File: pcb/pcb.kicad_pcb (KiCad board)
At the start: 2 copper layers, 108.7 x 45.2 mm, 22 parts, among them SW1 SW_Push, U1 ATmega32U4-AU, Y1 Crystal_GND24_Small

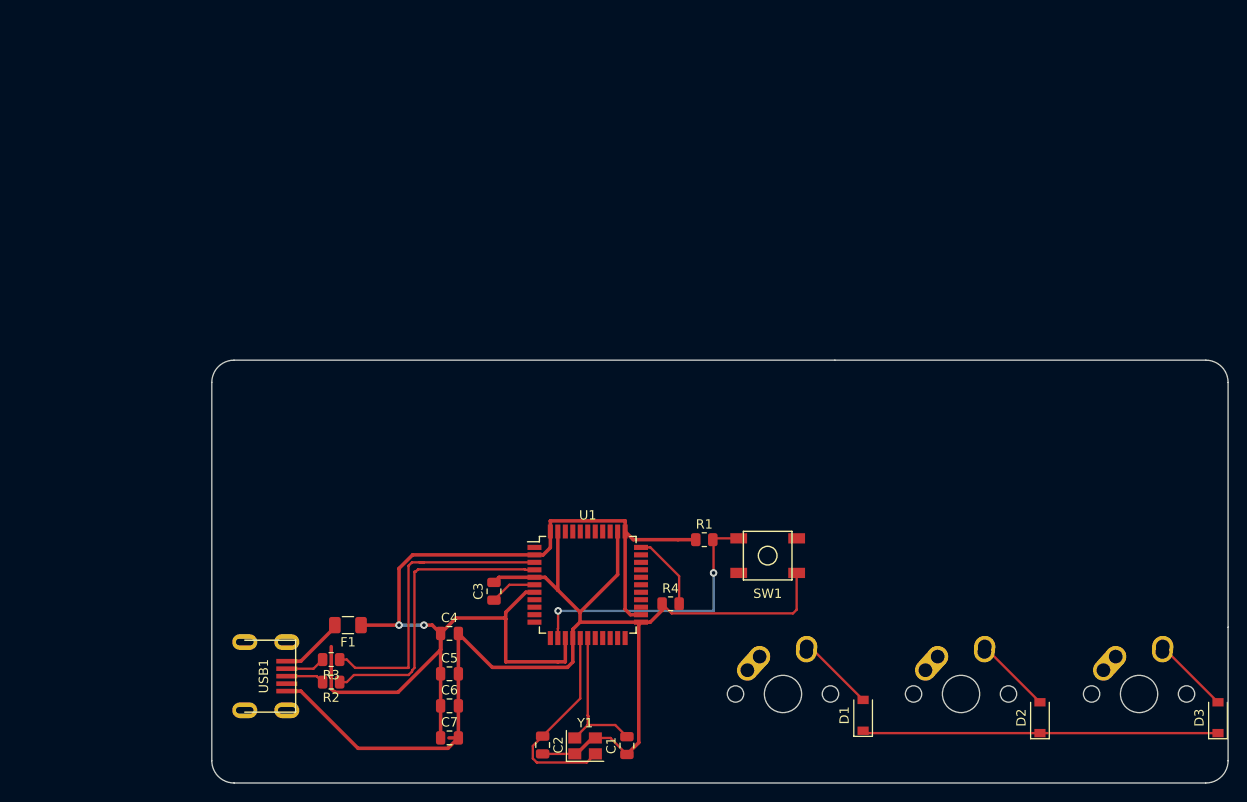
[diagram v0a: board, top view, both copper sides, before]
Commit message: finished tracing pcb
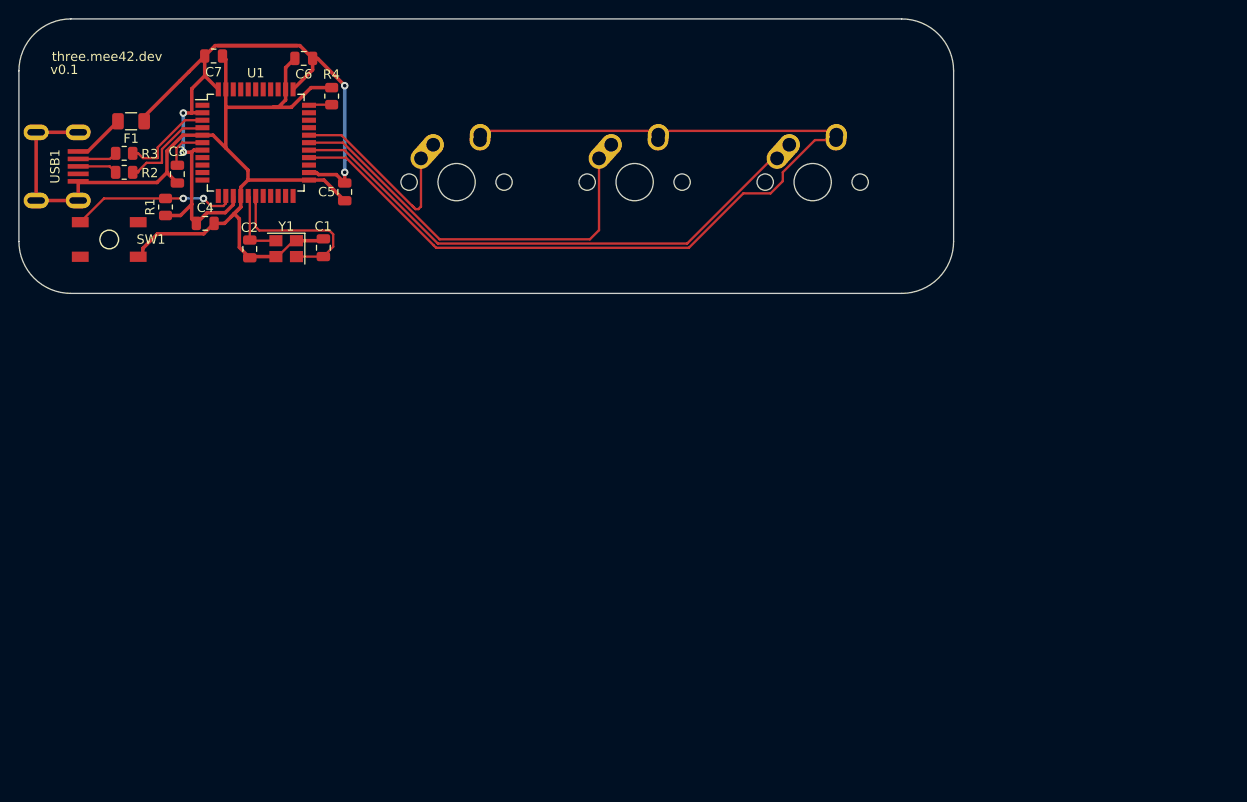
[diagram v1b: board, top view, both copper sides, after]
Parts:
- removed D1, D2, D3: D_Small, Diode_SMD:D_SOD-123
- moved SW1 78.2 mm to (24.7, 37.1)
- moved C7 77.2 mm to (35.9, 17.5)
- moved C6 71.0 mm to (45.6, 17.7), turned to 180 degrees
- moved R1 67.8 mm to (30.8, 33.6), turned to 90 degrees
- moved R4 65.3 mm to (48.5, 21.8), turned to 270 degrees
- moved MX1 65.0 mm to (61.9, 31.0)
- moved MX2 65.0 mm to (81.0, 31.0)
- moved MX3 65.0 mm to (100.0, 31.0)
- moved C1 62.4 mm to (47.7, 38.0), turned to 270 degrees
- moved Y1 62.1 mm to (43.7, 38.1), turned to 180 degrees
- moved C2 61.6 mm to (39.8, 38.1)
- moved U1 59.2 mm to (40.4, 26.7)
- moved USB1 58.9 mm to (16.9, 29.3)
- moved R2 58.9 mm to (26.3, 29.9)
- moved F1 58.7 mm to (27.1, 24.4)
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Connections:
- MX1 pad 2: Net-(D1-Pad2) -> ROW0
- MX2 pad 2: Net-(D2-Pad2) -> ROW0
- MX3 pad 2: Net-(D3-Pad2) -> ROW0
- U1 pad 26: Net-(U1-Pad26) -> ROW0
- U1 pad 27: Net-(U1-Pad27) -> COL2
- U1 pad 28: Net-(U1-Pad28) -> COL1
- U1 pad 29: Net-(U1-Pad29) -> COL0
- USB1 pad 6: Net-(USB1-Pad6) -> GND
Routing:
- net ROW0: track 38.1 -> 105.1 mm
- net COL2: track 0.00 -> 58.0 mm
- net COL1: track 0.00 -> 43.4 mm
- net +5V: track 119.3 -> 89.4 mm, vias 2 -> 4
- net Net-(R3-Pad1): track 32.8 -> 9.99 mm
- net Net-(R2-Pad1): track 32.0 -> 10.7 mm
- net COL0: track 0.00 -> 20.8 mm
- net GND: track 135.6 -> 116.9 mm
- net Net-(C2-Pad1): track 22.4 -> 7.61 mm
- net Net-(R1-Pad2): track 30.0 -> 17.9 mm
- net Net-(D1-Pad2): track 8.20 -> 0.00 mm
- net Net-(D3-Pad2): track 8.18 -> 0.00 mm
- net Net-(D2-Pad2): track 8.18 -> 0.00 mm
- net Net-(R4-Pad2): track 8.31 -> 2.45 mm
- net Net-(C1-Pad2): track 16.4 -> 18.5 mm
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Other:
- board size 108.7 x 45.2 mm -> 100 x 29.4 mm
- board text added: "three.mee42.dev"
- board text added: "v0.1"
